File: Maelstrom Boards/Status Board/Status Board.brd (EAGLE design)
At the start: 101.6 x 101.6 mm, 14 parts, among them P1 39-30-04?

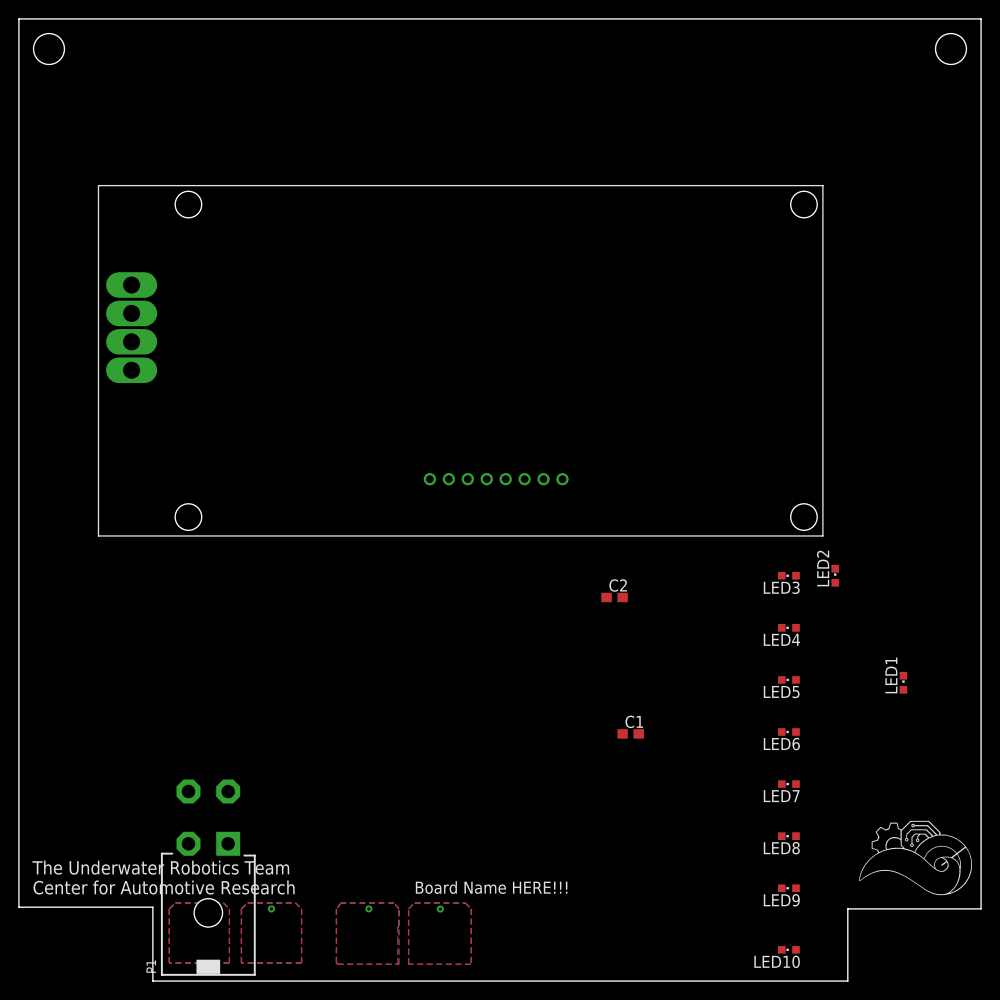
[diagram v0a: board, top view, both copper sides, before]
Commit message: Update Status Board
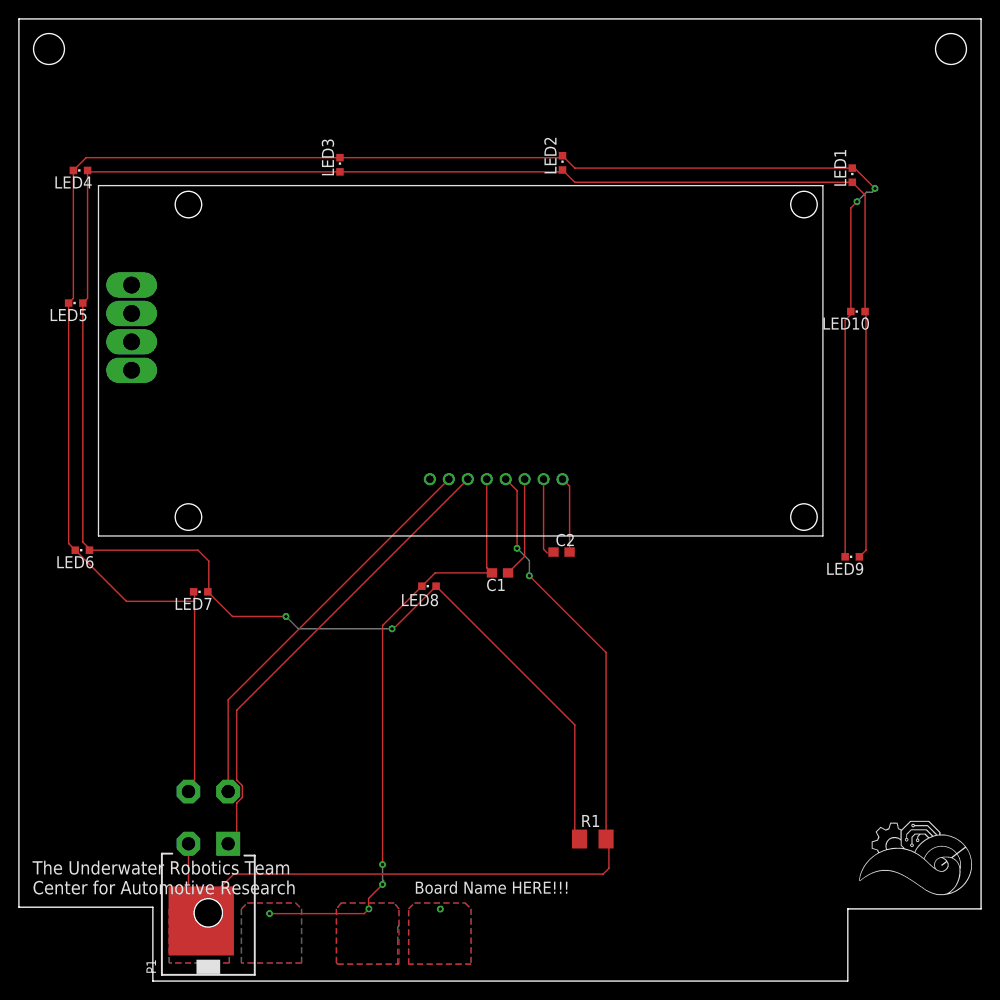
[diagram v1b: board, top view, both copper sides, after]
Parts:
- added R1: 23.333333, rcl:M3216
- moved LED4 89.0 mm to (6.50, 85.6)
- moved LED5 85.2 mm to (6.00, 71.6)
- moved LED6 77.0 mm to (6.70, 45.5)
- moved LED10 67.8 mm to (88.6, 70.7)
- moved LED7 65.3 mm to (19.2, 41.1)
- moved LED3 64.3 mm to (33.9, 86.2), turned to 0 degrees
- moved LED1 53.9 mm to (88.0, 85.1)
- moved LED2 52.3 mm to (57.4, 86.4)
- moved LED8 46.3 mm to (43.3, 41.7)
- moved LED9 35.6 mm to (88.0, 44.8)
- moved C1 21.9 mm to (50.8, 43.1), turned to 180 degrees
- moved C2 7.38 mm to (57.3, 45.3)
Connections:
- net +3V3: now also R1.2
- net N$4: now also R1.1
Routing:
- net GND: track 0.00 -> 268.5 mm, vias 2 -> 6
- net N$4: track 0.00 -> 238.2 mm, vias 0 -> 2
- net +3V3: track 0.00 -> 94.3 mm, vias 1 -> 3
- net SDA: track 0.00 -> 48.6 mm
- net SCL: track 0.00 -> 42.6 mm
- net N$3: track 0.00 -> 10.6 mm
- net N$2: track 0.00 -> 8.01 mm
- net N$1: track 0.00 -> 7.97 mm
